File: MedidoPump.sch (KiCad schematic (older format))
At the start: 47 parts, among them J1 Flow_Fwd, J2 Flow_Rev, J3 Flow_Stop, J4 MultiplexConn, J5 OLED Disp, J6 Press_Sens, J7 MultiplexConn, J8 PwrButton, Q1 2N3904, Q2 Q_PMOS_GDS, SW1 SW_DPST, SW2 On/Off, U1 Particle_Argon, U2 HEF4093B, U3 LM7805_TO220, U6 Pololu18v17

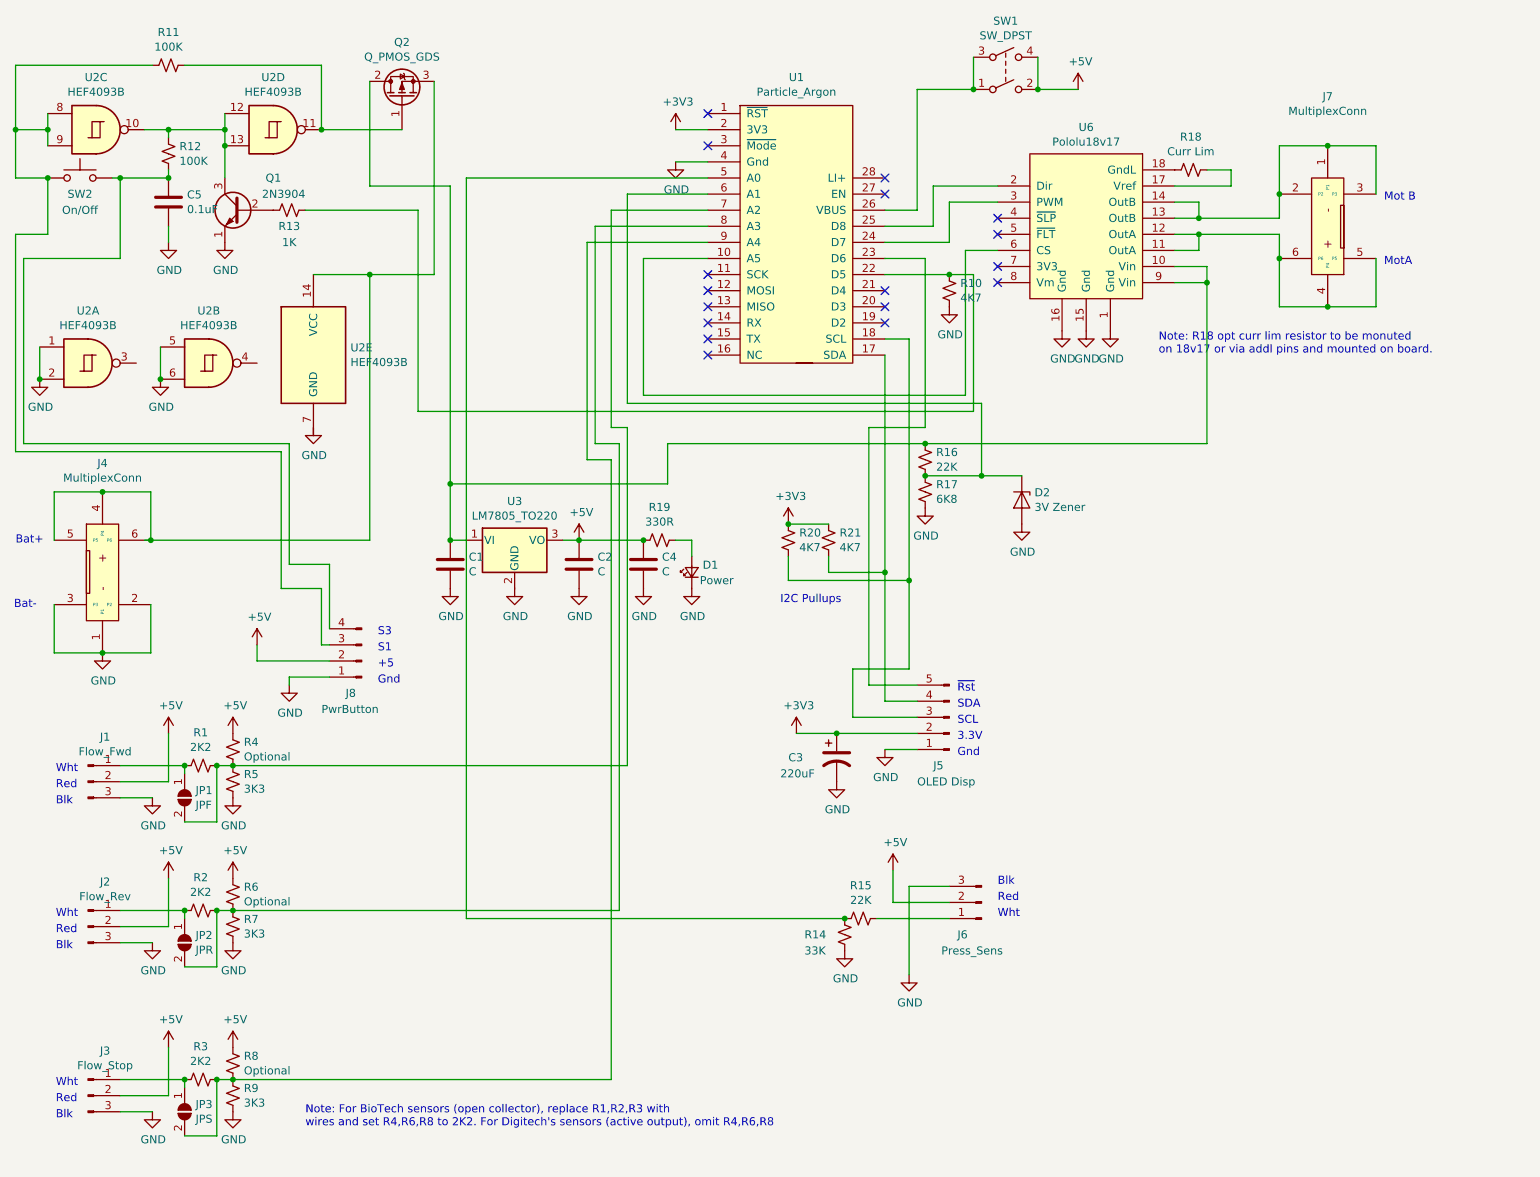
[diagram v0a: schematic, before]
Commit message: misc
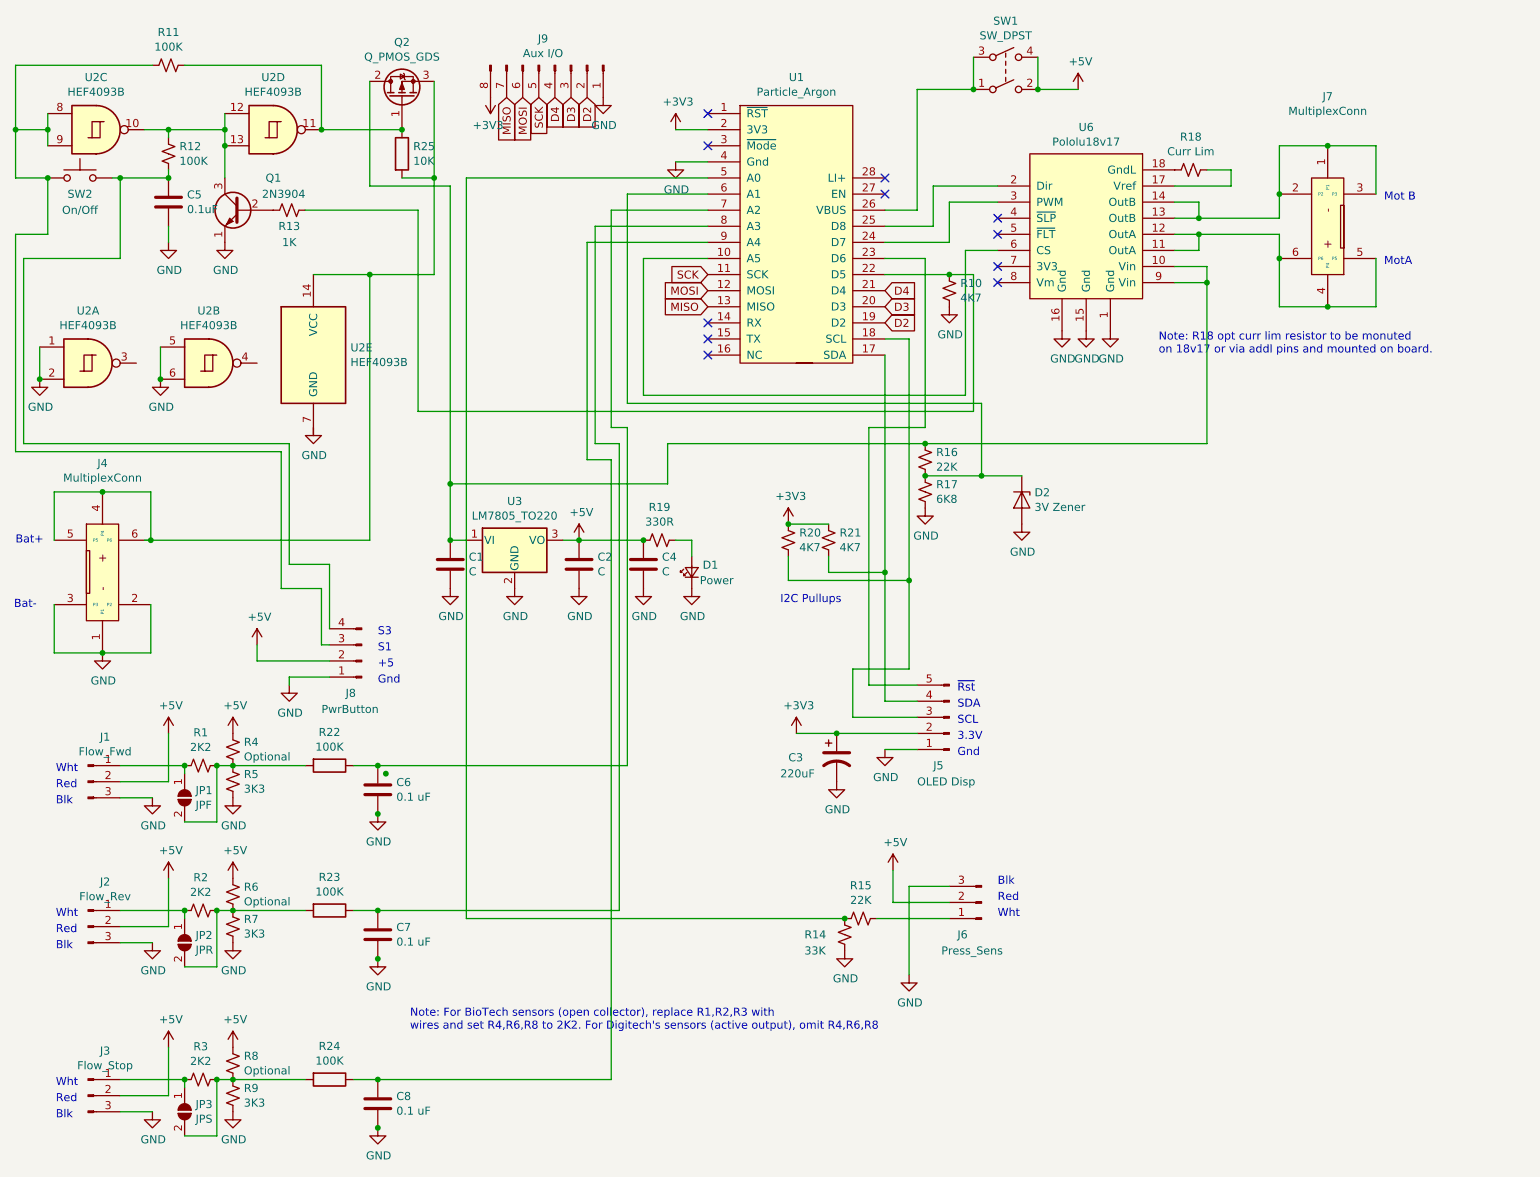
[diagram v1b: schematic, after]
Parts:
- added C6, C7, C8: 0.1 uF, Capacitor_THT:C_Disc_D12.0mm_W4.4mm_P7.75mm, symbol Device:C
- added J9: Aux I/O, Connector_PinHeader_2.54mm:PinHeader_1x08_P2.54mm_Vertical, symbol Connector:Conn_01x08_Male
- added R22, R23, R24: 100K, Resistor_THT:R_Axial_DIN0207_L6.3mm_D2.5mm_P10.16mm_Horizontal, symbol Device:R
- added R25: 10K, Resistor_THT:R_Axial_DIN0207_L6.3mm_D2.5mm_P10.16mm_Horizontal, symbol Device:R
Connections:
- net +3V3: now also J9.8 (Pin_8)
- net GND: now also C6.2, C7.2, C8.2, J9.1 (Pin_1)
- net at JP1.2 (B), R1.1, R4.2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: now also R22.2; no longer U1.7 (A2)
- net at JP2.2 (B), R2.1, R6.2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: now also R23.2; no longer U1.8 (A3)
- net at JP3.2 (B), R3.1, R8.2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: now also R24.2; no longer U1.9 (A4)
- net at J4.4 (P4), J4.5 (P5), J4.6 (P6)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: now also R25.2
- net SCK: now reaches U1.11 (SCK)
- net SCK: now also J9.5 (Pin_5)
- net MOSI: now reaches U1.12 (MOSI)
- net MOSI: now also J9.6 (Pin_6)
- net MISO: now reaches U1.13 (MISO)
- net MISO: now also J9.7 (Pin_7)
- net D2: now reaches U1.19 (D2)
- net D2: now also J9.2 (Pin_2)
- net D3: now reaches U1.20 (D3)
- net D3: now also J9.3 (Pin_3)
- net D4: now reaches U1.21 (D4)
- net D4: now also J9.4 (Pin_4)
- net at Q2.1 (G), R11.1, U2.11: now also R25.1
- new net: C6.1, R22.1, U1.7 (A2)
- new net: C7.1, R23.1, U1.8 (A3)
- new net: C8.1, R24.1, U1.9 (A4)
- no-connect marks 17 -> 11
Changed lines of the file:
@@
 Text Notes 900  7200 0    50   ~ 0
 Wht
-Wire Wire Line
-	4350 7150 2000 7150
-Wire Wire Line
-	4400 6100 2000 6100
-Wire Wire Line
-	4450 5200 2000 5200
 Text Notes 6750 5950 0    50   ~ 0
 Blk
@@
 	9100 2350 9100 2050
 Connection ~ 8800 2350
-Text Notes 2450 7450 0    50   ~ 0
+Text Notes 3100 6850 0    50   ~ 0
 Note: For BioTech sensors (open collector), replace R1,R2,R3 with \nwires and set R4,R6,R8 to 2K2. For Digitech's sensors (active output), omit R4,R6,R8\n
 $Comp
@@
 Wire Wire Line
 	4350 3300 4350 7150
-NoConn ~ 6050 2250
-NoConn ~ 6050 2350
-NoConn ~ 6050 2450
-NoConn ~ 4950 2150
-NoConn ~ 4950 2250
-NoConn ~ 4950 2350
 NoConn ~ 4950 2450
 NoConn ~ 4950 2550
@@
 Connection ~ 3350 3450
 Wire Wire Line
-	3250 950  3250 2150
+	3250 950  3250 1550
 Wire Wire Line
 	3250 2150 2850 2150
@@
 	1900 7500 1900 7150
 Connection ~ 1900 7150
+$Comp
+L Device:R R22
+U 1 1 602B8F57
+P 2600 5200
+F 0 "R22" V 2393 5200 50  0000 C CNN
+F 1 "100K" V 2484 5200 50  0000 C CNN
+F 2 "Resistor_THT:R_Axial_DIN0207_L6.3mm_D2.5mm_P10.16mm_Horizontal" V 2530 5200 50  0001 C CNN
+F 3 "~" H 2600 5200 50  0001 C CNN
+	1    2600 5200
+	0    1    1    0
+$EndComp
+Wire Wire Line
+	2750 5200 2900 5200
+Wire Wire Line
+	2000 5200 2450 5200
+$Comp
+L Device:C C6
+U 1 1 602CF131
+P 2900 5350
+F 0 "C6" H 3015 5396 50  0000 L CNN
+F 1 "0.1 uF" H 3015 5305 50  0000 L CNN
+F 2 "Capacitor_THT:C_Disc_D12.0mm_W4.4mm_P7.75mm" H 2938 5200 50  0001 C CNN
+F 3 "~" H 2900 5350 50  0001 C CNN
+	1    2900 5350
+	1    0    0    -1
+$EndComp
+Connection ~ 2900 5200
+Wire Wire Line
+	2900 5200 4450 5200
+$Comp
+L Device:R R23
+U 1 1 602CF3C9
+P 2600 6100
+F 0 "R23" V 2393 6100 50  0000 C CNN
+F 1 "100K" V 2484 6100 50  0000 C CNN
+F 2 "Resistor_THT:R_Axial_DIN0207_L6.3mm_D2.5mm_P10.16mm_Horizontal" V 2530 6100 50  0001 C CNN
+F 3 "~" H 2600 6100 50  0001 C CNN
+	1    2600 6100
+	0    1    1    0
+$EndComp
+Wire Wire Line
+	2000 6100 2450 6100
+Wire Wire Line
+	2750 6100 2900 6100
+$Comp
+L Device:C C7
+U 1 1 602E5EE6
+P 2900 6250
+F 0 "C7" H 3015 6296 50  0000 L CNN
+F 1 "0.1 uF" H 3015 6205 50  0000 L CNN
+F 2 "Capacitor_THT:C_Disc_D12.0mm_W4.4mm_P7.75mm" H 2938 6100 50  0001 C CNN
+F 3 "~" H 2900 6250 50  0001 C CNN
+	1    2900 6250
+	1    0    0    -1
+$EndComp
+Connection ~ 2900 6100
+Wire Wire Line
+	2900 6100 4400 6100
+$Comp
+L power:GND #PWR031
+U 1 1 602E5FDD
+P 2900 6400
+F 0 "#PWR031" H 2900 6150 50  0001 C CNN
+F 1 "GND" H 2905 6227 50  0000 C CNN
+F 2 "" H 2900 6400 50  0001 C CNN
+F 3 "" H 2900 6400 50  0001 C CNN
+	1    2900 6400
+	1    0    0    -1
+$EndComp
+$Comp
+L Device:R R24
+U 1 1 602E6119
+P 2600 7150
+F 0 "R24" V 2393 7150 50  0000 C CNN
+F 1 "100K" V 2484 7150 50  0000 C CNN
+F 2 "Resistor_THT:R_Axial_DIN0207_L6.3mm_D2.5mm_P10.16mm_Horizontal" V 2530 7150 50  0001 C CNN
+F 3 "~" H 2600 7150 50  0001 C CNN
+	1    2600 7150
+	0    1    1    0
+$EndComp
+$Comp
+L Device:C C8
+U 1 1 602E6253
+P 2900 7300
+F 0 "C8" H 3015 7346 50  0000 L CNN
+F 1 "0.1 uF" H 3015 7255 50  0000 L CNN
+F 2 "Capacitor_THT:C_Disc_D12.0mm_W4.4mm_P7.75mm" H 2938 7150 50  0001 C CNN
+F 3 "~" H 2900 7300 50  0001 C CNN
+	1    2900 7300
+	1    0    0    -1
+$EndComp
+$Comp
+L power:GND #PWR032
+U 1 1 602E63C4
+P 2900 7450
+F 0 "#PWR032" H 2900 7200 50  0001 C CNN
+F 1 "GND" H 2905 7277 50  0000 C CNN
+F 2 "" H 2900 7450 50  0001 C CNN
+F 3 "" H 2900 7450 50  0001 C CNN
+	1    2900 7450
+	1    0    0    -1
+$EndComp
+Wire Wire Line
+	2000 7150 2450 7150
+Wire Wire Line
+	2750 7150 2900 7150
+Connection ~ 2900 7150
+Wire Wire Line
+	2900 7150 4350 7150
+Text GLabel 6050 2250 2    50   Input ~ 0
+D4
+Text GLabel 6050 2350 2    50   Input ~ 0
+D3
+Text GLabel 6050 2450 2    50   Input ~ 0
+D2
+Text GLabel 4950 2150 0    50   Input ~ 0
+SCK
+Text GLabel 4950 2250 0    50   Input ~ 0
+MOSI
+Text GLabel 4950 2350 0    50   Input ~ 0
+MISO
+$Comp
+L Connector:Conn_01x08_Male J9
+U 1 1 60316BF7
+P 4000 850
+F 0 "J9" V 3835 776 50  0000 C CNN
+F 1 "Aux I/O" V 3926 776 50  0000 C CNN
+F 2 "Connector_PinHeader_2.54mm:PinHeader_1x08_P2.54mm_Vertical" H 4000 850 50  0001 C CNN
+F 3 "~" H 4000 850 50  0001 C CNN
+	1    4000 850
+	0    1    1    0
+$EndComp
+$Comp
+L power:GND #PWR036
+U 1 1 60316EB2
+P 4300 1050
+F 0 "#PWR036" H 4300 800 50  0001 C CNN
+F 1 "GND" H 4305 877 50  0000 C CNN
+F 2 "" H 4300 1050 50  0001 C CNN
+F 3 "" H 4300 1050 50  0001 C CNN
+	1    4300 1050
+	1    0    0    -1
+$EndComp
+$Comp
+L power:+3V3 #PWR034
+U 1 1 60316FC5
+P 3600 1050
+F 0 "#PWR034" H 3600 900 50  0001 C CNN
+F 1 "+3V3" H 3615 1223 50  0000 C CNN
+F 2 "" H 3600 1050 50  0001 C CNN
+F 3 "" H 3600 1050 50  0001 C CNN
+	1    3600 1050
+	-1   0    0    1
+$EndComp
+Text GLabel 4200 1050 3    50   Input ~ 0
+D2
+Text GLabel 4100 1050 3    50   Input ~ 0
+D3
+Text GLabel 4000 1050 3    50   Input ~ 0
+D4
+Text GLabel 3900 1050 3    50   Input ~ 0
+SCK
+Text GLabel 3800 1050 3    50   Input ~ 0
+MOSI
+Text GLabel 3700 1050 3    50   Input ~ 0
+MISO
+$Comp
+L Device:R R25
+U 1 1 603178CB
+P 3050 1400
+F 0 "R25" H 3120 1446 50  0000 L CNN
+F 1 "10K" H 3120 1355 50  0000 L CNN
+F 2 "Resistor_THT:R_Axial_DIN0207_L6.3mm_D2.5mm_P10.16mm_Horizontal" V 2980 1400 50  0001 C CNN
+F 3 "~" H 3050 1400 50  0001 C CNN
+	1    3050 1400
+	1    0    0    -1
+$EndComp
+Connection ~ 3050 1250
+Wire Wire Line
+	3050 1550 3250 1550
+Connection ~ 3250 1550
+Wire Wire Line
+	3250 1550 3250 2150
+$Comp
+L power:GND #PWR0102
+U 1 1 603264A9
+P 2900 5500
+F 0 "#PWR0102" H 2900 5250 50  0001 C CNN
+F 1 "GND" H 2905 5327 50  0000 C CNN
+F 2 "" H 2900 5500 50  0001 C CNN
+F 3 "" H 2900 5500 50  0001 C CNN
+	1    2900 5500
+	1    0    0    -1
+$EndComp
+Connection ~ 2900 5500
+Connection ~ 2900 6400
+Connection ~ 2900 7450
+Connection ~ 2950 5250
 $EndSCHEMATC
